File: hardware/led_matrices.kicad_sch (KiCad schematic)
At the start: 280 parts

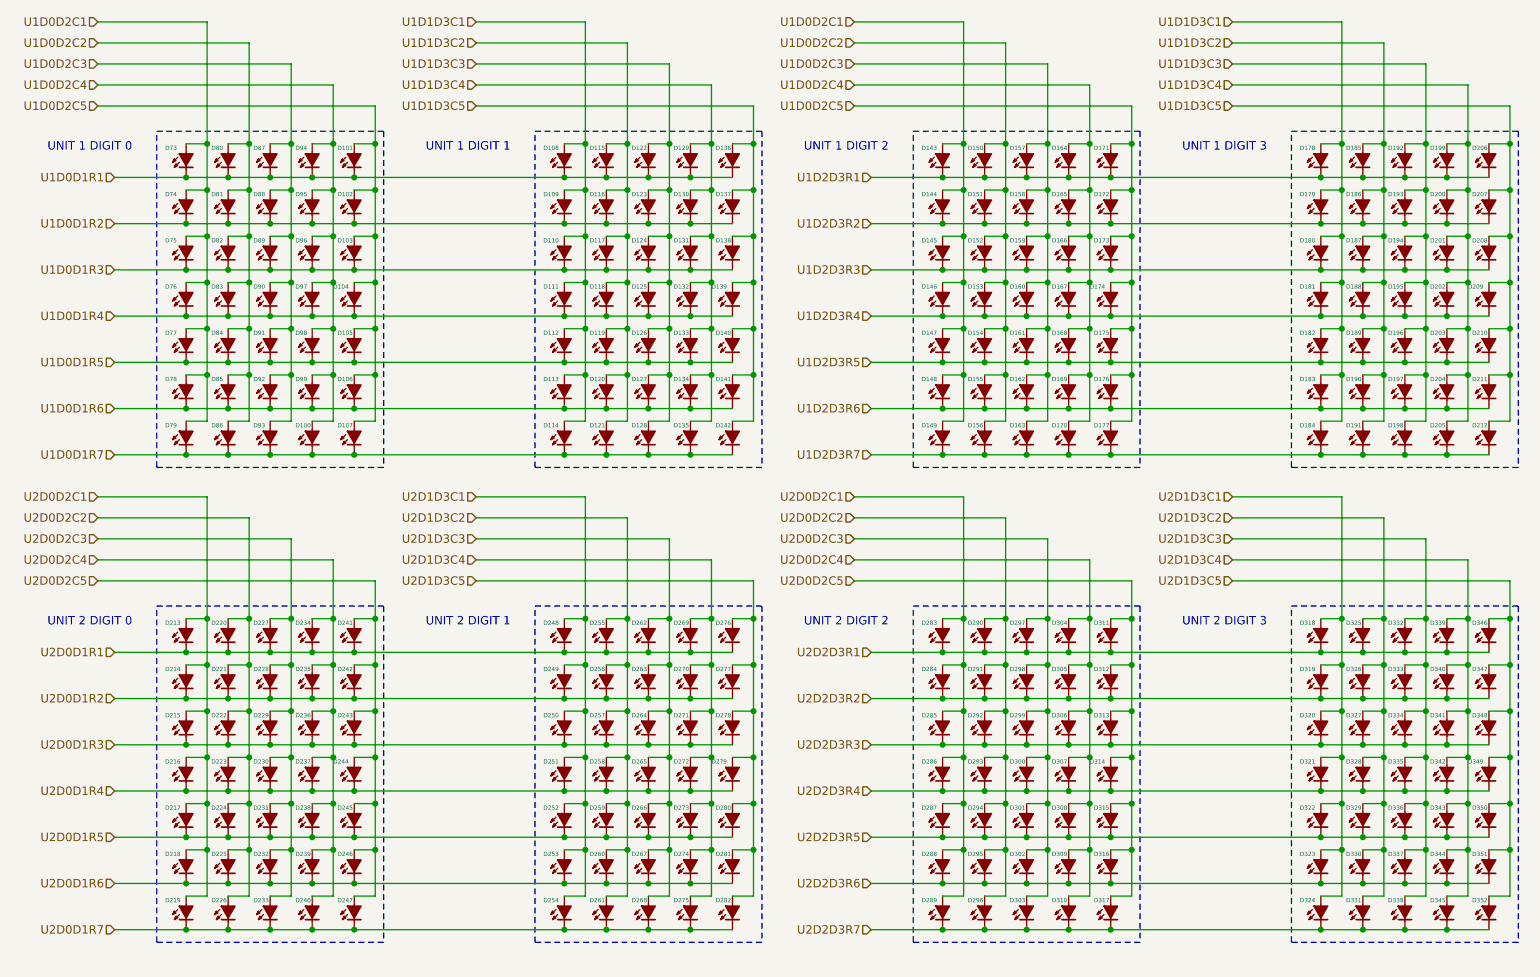
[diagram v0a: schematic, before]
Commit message: Starting PCB routing process
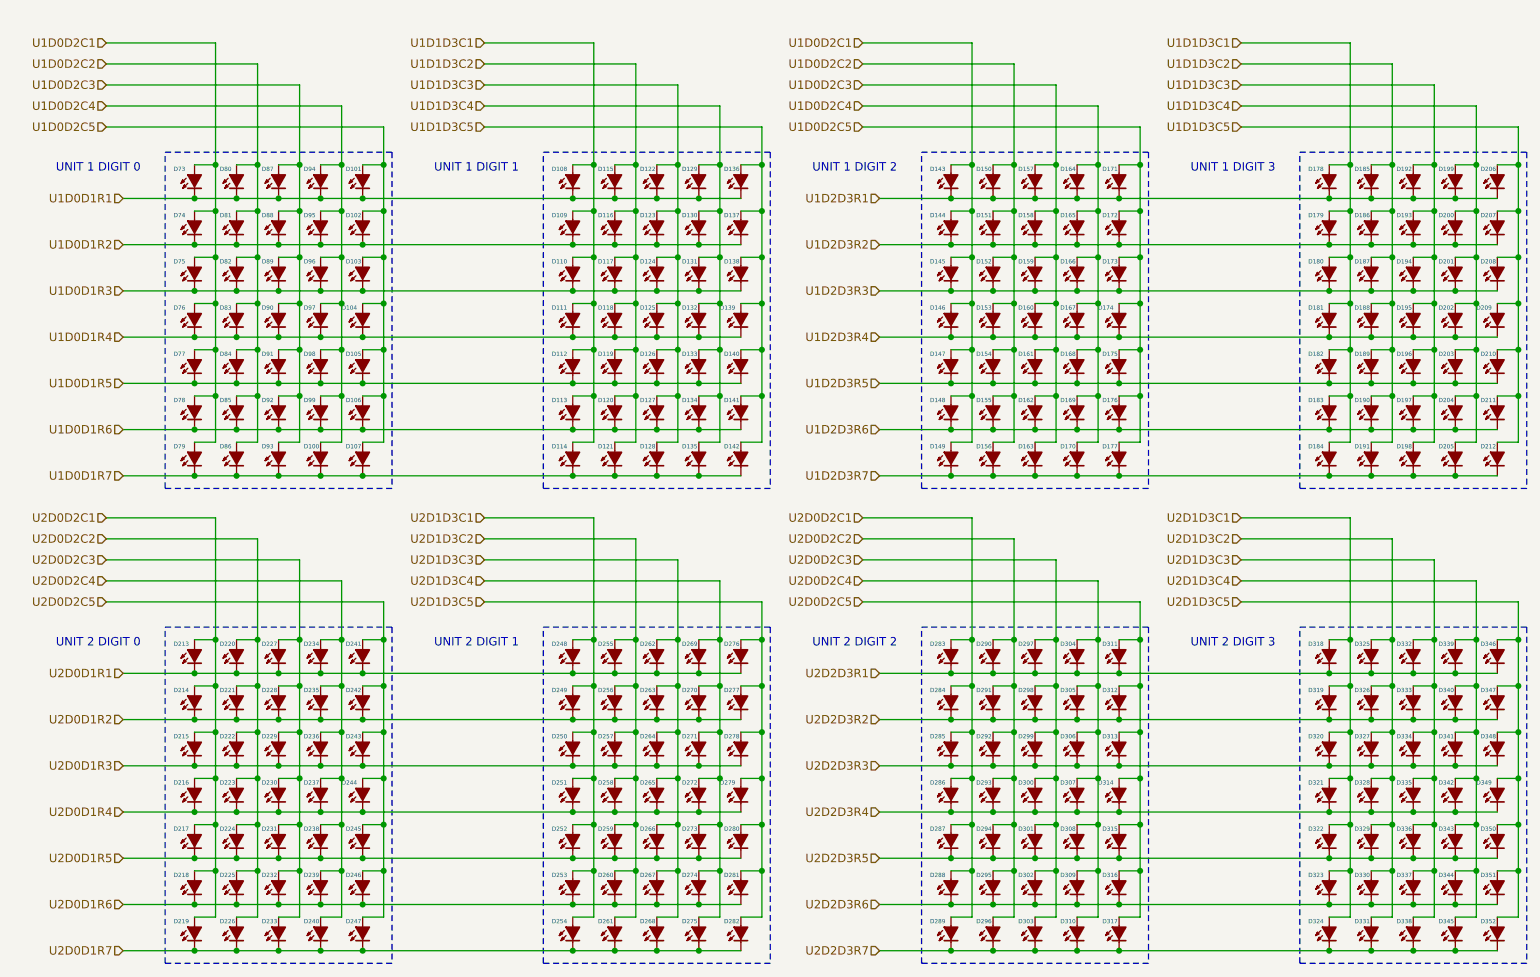
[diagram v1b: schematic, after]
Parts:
- D100, D101, D102, D103, D104, D105, D106, D107, D108, D109, D110, D111, D112, D113, D114, D115, D116, D117, D118, D119, D120, D121, D122, D123, D124, D125, D126, D127, D128, D129, D130, D131, D132, D133, D134, D135, D136, D137, D138, D139, D140, D141, D142, D143, D144, D145, D146, D147, D148, D149, D150, D151, D152, D153, D154, D155, D156, D157, D158, D159, D160, D161, D162, D163, D164, D165, D166, D167, D168, D169, D170, D171, D172, D173, D174, D175, D176, D177, D178, D179, D180, D181, D182, D183, D184, D185, D186, D187, D188, D189, D190, D191, D192, D193, D194, D195, D196, D197, D198, D199, D200, D201, D202, D203, D204, D205, D206, D207, D208, D209, D210, D211, D212, D73, D74, D75, D76, D77, D78, D79, D80, D81, D82, D83, D84, D85, D86, D87, D88, D89, D90, D91, D92, D93, D94, D95, D96, D97, D98, D99: footprint LED_THT_espena:LED_D3.0mm_p2.28 -> LED_THT_espena:LED_D5.0mm_p2.54
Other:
- moved on the sheet: D100, D101, D102, D103, D104, D105, D106, D107, D108, D109, D110, D111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
